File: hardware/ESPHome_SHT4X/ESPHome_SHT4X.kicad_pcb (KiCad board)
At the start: 2 copper layers, 50 x 30.6 mm, 43 parts, among them J2 UJ20-C-H-G-SMT-2A-P16-TR, SW1 SW_Push, SW2 SW_Push, SW3 SW_Push, U1 ESP32-C6-WROOM-1-N8, U2 BQ25628ERYKR, U3 SHT40-AD1F-R2, U4 XC6220B331MR-G

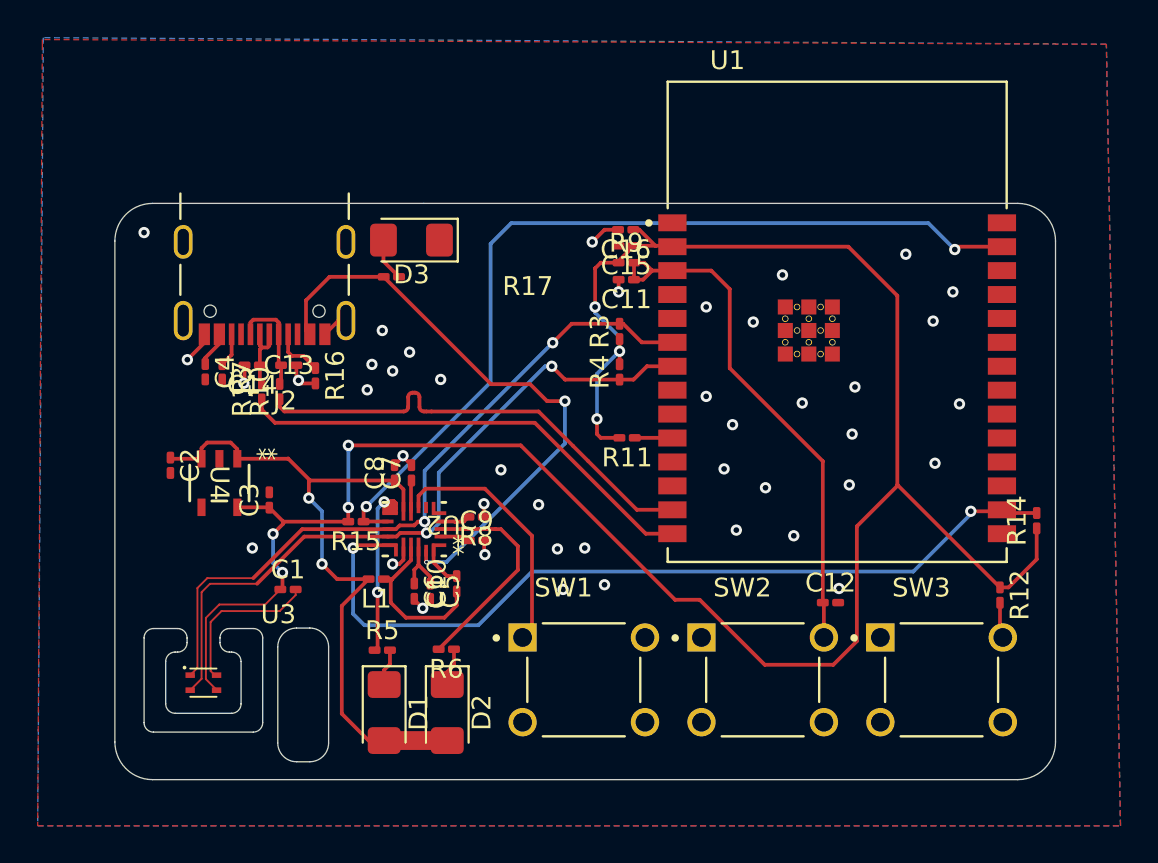
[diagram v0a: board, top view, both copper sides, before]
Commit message: making more progress
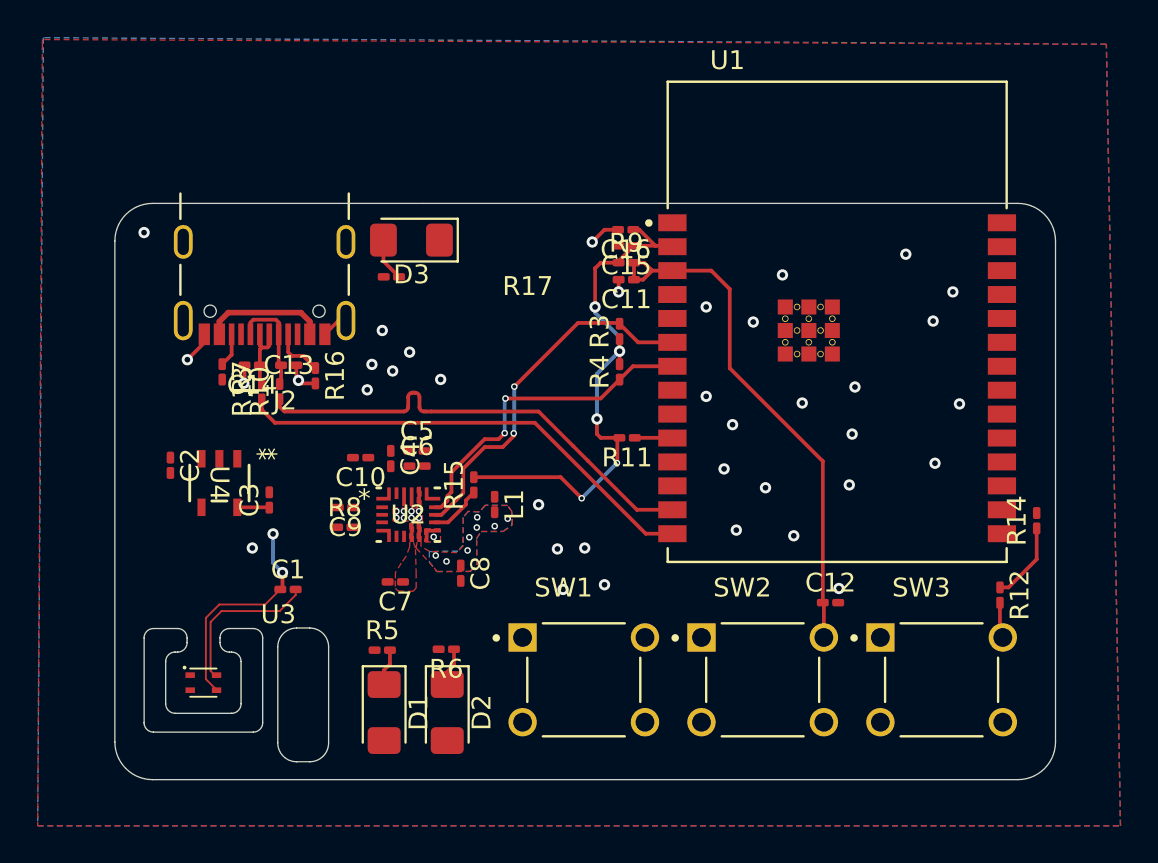
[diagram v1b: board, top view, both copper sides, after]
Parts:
- U2: footprint Library:WQFN-HR18__RYK_TEX -> ESPhome:WQFN-HR18__RYK_TEX
- moved C4 10.9 mm to (144.5, 68.8)
- moved C10 8.42 mm to (142.9, 68.7), turned to 180 degrees
- moved C5 7.48 mm to (145.9, 68.3), turned to 0 degrees
- moved L1 7.43 mm to (150.0, 71.2), turned to -90 degrees
- moved C9 7.17 mm to (142.1, 71.3), turned to 180 degrees
- moved R8 7.00 mm to (142.1, 72.4), turned to 0 degrees
- moved C6 6.64 mm to (145.9, 69.2), turned to 0 degrees
- moved R15 6.56 mm to (148.9, 70.1), turned to 90 degrees
- moved C8 6.39 mm to (148.2, 74.8), turned to -90 degrees
- moved C7 5.86 mm to (144.7, 75.3), turned to 180 degrees
- moved U2 0.83 mm to (145.4, 71.7), turned to 0 degrees
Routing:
- net ESP_3V3: track 118.3 -> 46.7 mm
- net IO18: track 45.1 -> 0.00 mm, vias 2 -> 0
- net *INT: track 47.1 -> 2.86 mm, vias 2 -> 0
- net SYS: track 37.1 -> 0.00 mm, vias 2 -> 8
- net VBUS: track 33.6 -> 6.54 mm, vias 2 -> 0
- net SCL: track 37.6 -> 17.5 mm
- net SDA: track 37.9 -> 19.7 mm
- net Net-(U2-STAT): track 13.9 -> 0.00 mm, vias 2 -> 1
- net *QON: track 13.4 -> 0.00 mm
- net Net-(U2-*PG): track 11.7 -> 0.00 mm
- net SW: track 8.67 -> 0.00 mm
- net GND: track 22.3 -> 16.8 mm, vias 43 -> 45
- net PMID: track 3.28 -> 0.00 mm
- net BTST: track 2.45 -> 0.00 mm
- net BAT: track 1.65 -> 0.00 mm
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- added copper zone on F.Cu, net BAT
- added copper zone on F.Cu, net Net-(U2-STAT)
- added copper zone on B.Cu, net SYS
- added copper zone on F.Cu, net SYS
